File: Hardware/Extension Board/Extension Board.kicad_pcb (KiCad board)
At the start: 2 copper layers, 48.3 x 100 mm, 34 parts, among them J1 CNX_LED, J10 CNX_MODE, J11 CNX_TUNING, J12 CNX_I2C, J13 CNX_I2C, J14 CNX_SPI, J15 CNX_SD, J16 CNX_TFT, J2 CNX_LED, J3 CNX_LED, J4 CNX_LED, J5 CNX_SPARE, J6 ARDUINO_DIGITAL, J7 ARDUINO_COMMS, J8 ARDUINO_ANALOG, J9 CNX_NEXT_AGAIN, U1 74HC14

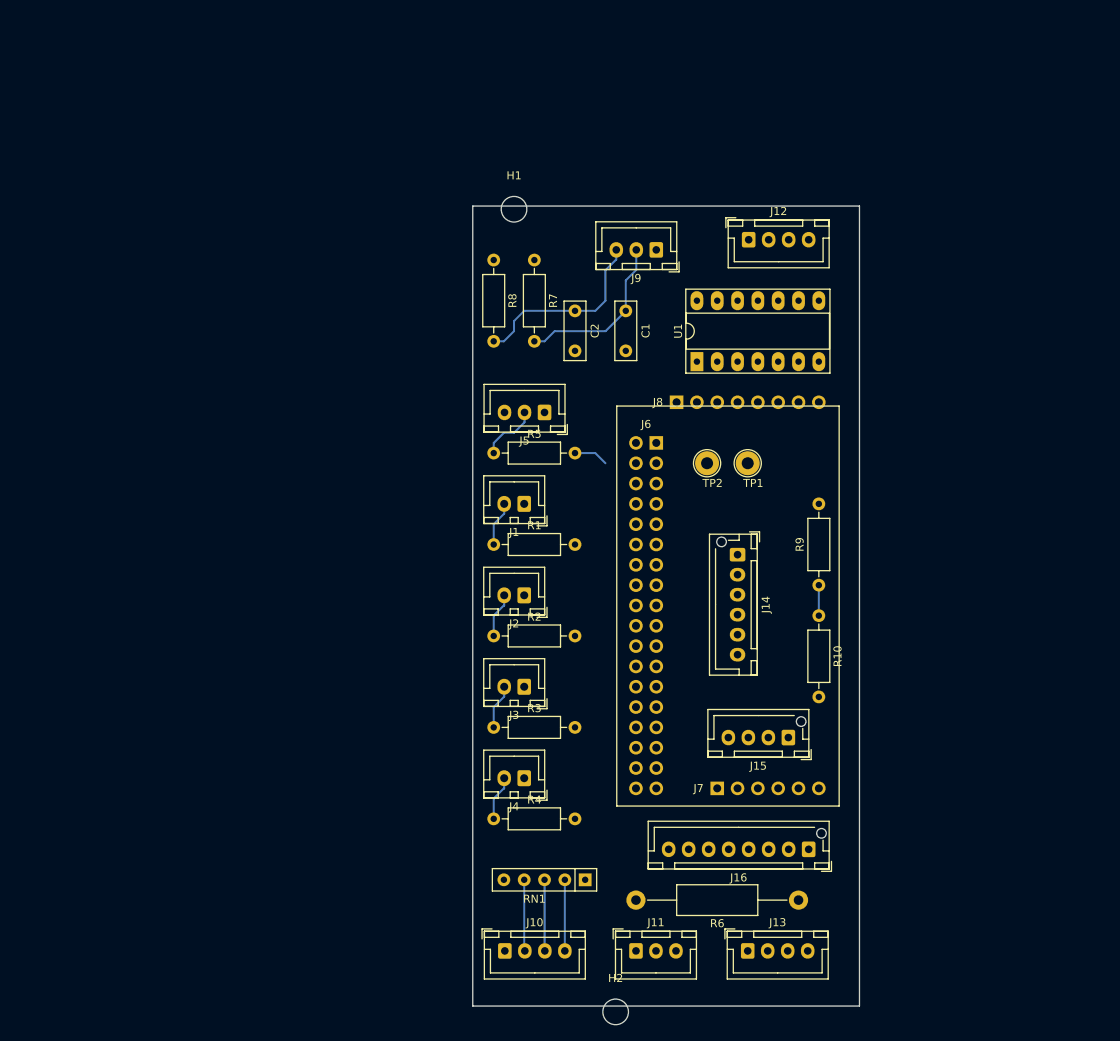
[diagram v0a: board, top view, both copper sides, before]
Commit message: PCB Extension board
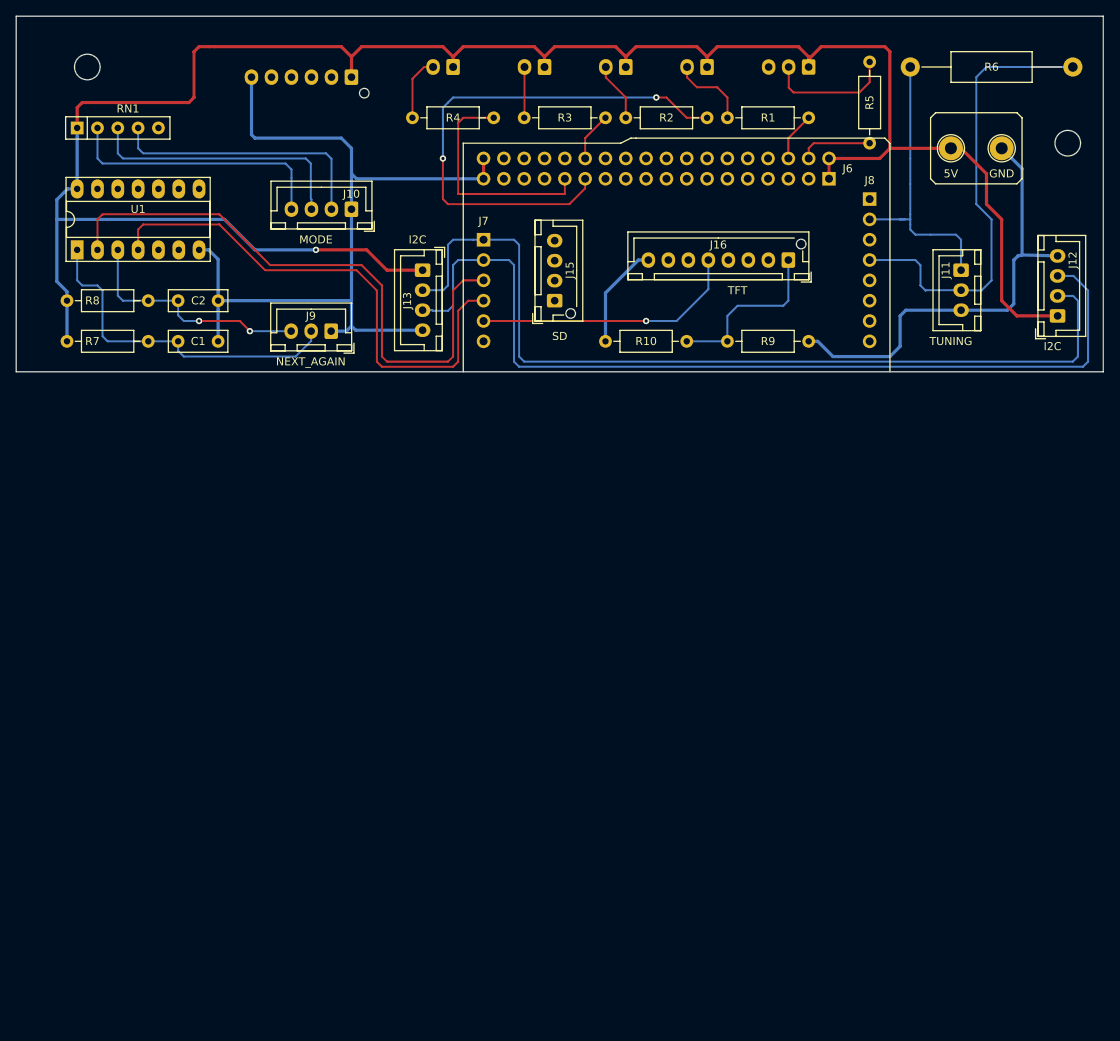
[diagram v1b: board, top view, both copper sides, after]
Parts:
- J1, J2, J3, J4: moved to B.Cu
- J10: value CNX_MODE -> MODE
- J11: value CNX_TUNING -> TUNING
- J12, J13: value CNX_I2C -> I2C
- J14: value CNX_SPI -> SPI; moved to B.Cu
- J15: value CNX_SD -> SD
- J16: value CNX_TFT -> TFT
- J5: value CNX_SPARE -> SPARE; moved to B.Cu
- J9: value CNX_NEXT_AGAIN -> NEXT_AGAIN
- moved H2 135.3 mm to (34.3, 44.5), turned to 180 degrees
- moved RN1 113.4 mm to (33.0, 52.1), turned to 0 degrees
- moved R6 109.6 mm to (157.5, 44.5)
- moved J10 94.7 mm to (67.3, 62.2), turned to 180 degrees
- moved J13 94.3 mm to (76.2, 69.8), turned to 270 degrees
- moved J11 94.3 mm to (143.5, 69.8), turned to 270 degrees
- moved J4 89.3 mm to (80.0, 44.5)
- moved R4 88.2 mm to (74.9, 50.8)
- moved U1 78.7 mm to (33.0, 67.3)
- moved J3 77.5 mm to (91.4, 44.5)
- moved J14 76.8 mm to (67.3, 45.7), turned to 180 degrees
- moved R3 76.3 mm to (88.9, 50.8)
- moved J7 74.5 mm to (83.8, 66.0), turned to 180 degrees
- moved J16 73.7 mm to (121.9, 68.6)
- moved H1 69.7 mm to (156.8, 54.0), turned to 180 degrees
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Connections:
- U1 pad 2: D18 -> D19
- U1 pad 4: D19 -> D18
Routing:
- net VCC: track 0.00 -> 278.2 mm, vias 0 -> 1
- net GND: track 0.00 -> 160.6 mm
- net SDA: track 0.00 -> 115.1 mm
- net SCL: track 0.00 -> 112.0 mm
- net D19: track 0.00 -> 74.2 mm
- net D44: track 0.00 -> 66.1 mm, vias 0 -> 2
- net D18: track 0.00 -> 65.7 mm
- net A12: track 0.00 -> 57.6 mm
- net A14: track 0.00 -> 36.7 mm
- net D17: track 0.00 -> 33.4 mm, vias 0 -> 1
- net D46: track 0.00 -> 28.8 mm
- net D33: track 8.89 -> 33.6 mm
- net D31: track 8.91 -> 33.6 mm
- net D29: track 8.92 -> 33.6 mm
- net Net-(C1-Pad1): track 21.2 -> 43.1 mm
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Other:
- board size 48.3 x 100 mm -> 135.9 x 44.4 mm
- net class Power added: clearance 0.2, trace_width 0.4, via_dia 0.8, via_drill 0.4
- board text added: "5V"
- board text added: "GND"
- board text added: "LEDs"
- board text added: "SPARE"
